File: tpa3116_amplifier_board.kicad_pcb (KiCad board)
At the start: 2 copper layers, 60.3 x 50.8 mm, 41 parts, among them IC1 TPA3116D2QDADRQ1, J1 power_supply, J2 Conn_01x04, J3 power_supply, J4 output_right

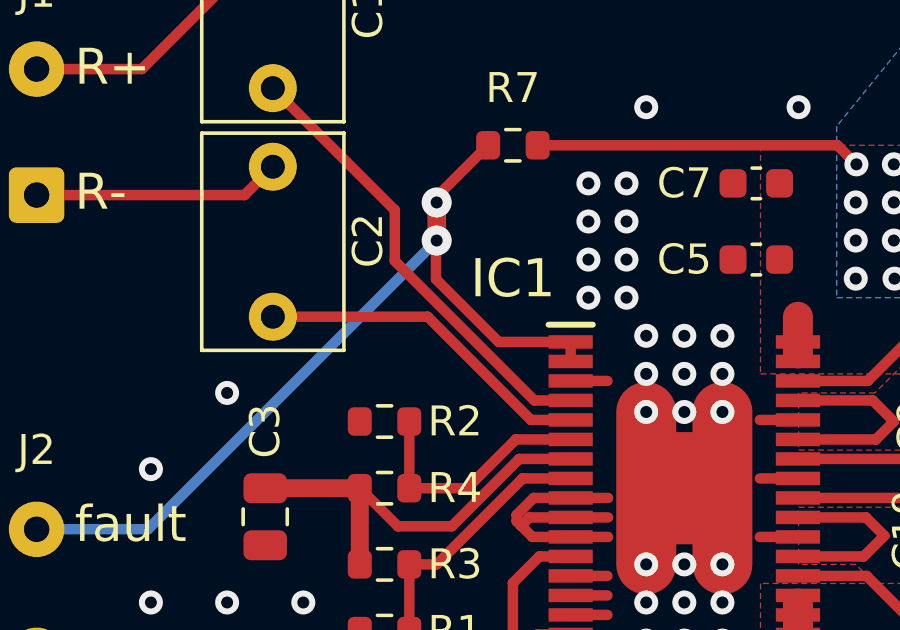
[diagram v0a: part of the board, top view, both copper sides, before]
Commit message: исправил ошибку в схеме
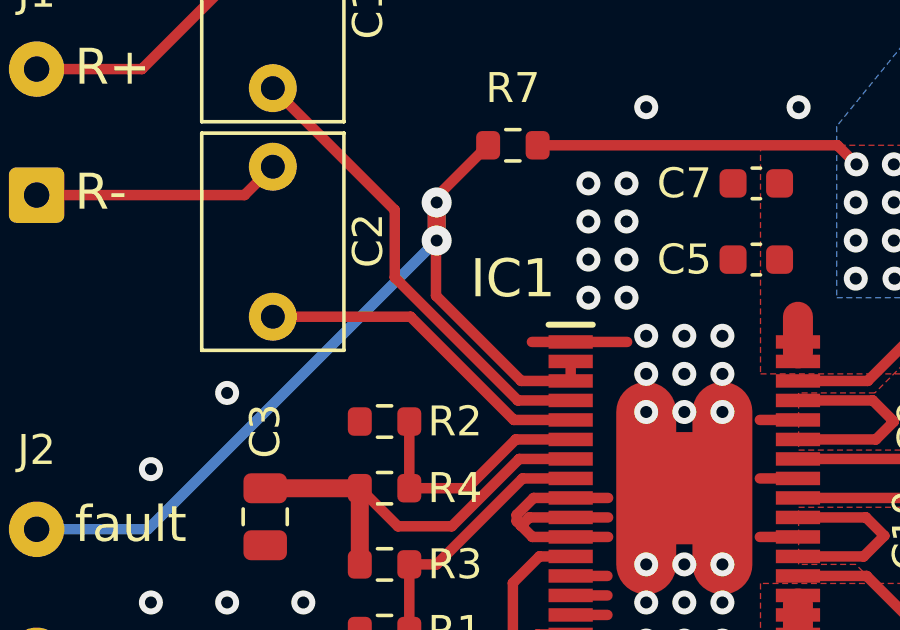
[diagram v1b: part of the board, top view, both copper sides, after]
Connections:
- IC1 pad 1: /SD_LR -> GND
- IC1 pad 3: GND -> /SD_LR
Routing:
- net GND: track 35.0 -> 36.9 mm
- net /SD_LR: track 29.8 -> 30.6 mm
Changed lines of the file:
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@@
       (stroke (width 0.1) (type solid)) (layer "F.Fab"))
     (pad "1" smd rect (at -3.788 -4.875 90) (size 0.45 1.475) (layers "F.Cu" "F.Paste" "F.Mask")
-      (net 16 "/SD_LR") (pinfunction "MODSEL") (pintype "passive"))
+      (net 5 "GND") (pinfunction "MODSEL") (pintype "passive"))
     (pad "2" smd rect (at -3.788 -4.225 90) (size 0.45 1.475) (layers "F.Cu" "F.Paste" "F.Mask")
       (net 16 "/SD_LR") (pinfunction "SD") (pintype "passive"))
     (pad "3" smd rect (at -3.788 -3.575 90) (size 0.45 1.475) (layers "F.Cu" "F.Paste" "F.Mask")
-      (net 5 "GND") (pinfunction "FAULT") (pintype "passive"))
+      (net 16 "/SD_LR") (pinfunction "FAULT") (pintype "passive"))
     (pad "4" smd rect (at -3.788 -2.925 90) (size 0.45 1.475) (layers "F.Cu" "F.Paste" "F.Mask")
       (net 2 "Net-(IC1-RINP)") (pinfunction "RINP") (pintype "passive"))
@@
   (segment (start 106.379 106.045) (end 102.87 106.045) (width 0.35) (layer "F.Cu") (net 1))
   (segment (start 110.744 101.68) (end 106.379 106.045) (width 0.35) (layer "F.Cu") (net 1))
-  (segment (start 120.672 117.09) (end 119.459831 117.09) (width 0.35) (layer "F.Cu") (net 2))
-  (segment (start 114.808 112.438169) (end 114.808 110.744) (width 0.35) (layer "F.Cu") (net 2))
-  (segment (start 119.459831 117.09) (end 114.808 112.438169) (width 0.35) (layer "F.Cu") (net 2))
+  (segment (start 118.909915 117.09) (end 114.808 112.988085) (width 0.35) (layer "F.Cu") (net 2))
   (segment (start 114.808 110.744) (end 110.744 106.68) (width 0.35) (layer "F.Cu") (net 2))
+  (segment (start 120.672 117.09) (end 118.909915 117.09) (width 0.35) (layer "F.Cu") (net 2))
+  (segment (start 114.808 112.988085) (end 114.808 110.744) (width 0.35) (layer "F.Cu") (net 2))
   (segment (start 102.87 110.245) (end 109.799 110.245) (width 0.35) (layer "F.Cu") (net 3))
   (segment (start 109.799 110.245) (end 110.744 109.3) (width 0.35) (layer "F.Cu") (net 3))
-  (segment (start 119.346155 117.74) (end 115.906155 114.3) (width 0.35) (layer "F.Cu") (net 4))
-  (segment (start 120.672 117.74) (end 119.346155 117.74) (width 0.35) (layer "F.Cu") (net 4))
-  (segment (start 115.906155 114.3) (end 110.744 114.3) (width 0.35) (layer "F.Cu") (net 4))
+  (segment (start 118.776538 117.74) (end 115.336538 114.3) (width 0.35) (layer "F.Cu") (net 4))
+  (segment (start 120.672 117.74) (end 118.776538 117.74) (width 0.35) (layer "F.Cu") (net 4))
+  (segment (start 115.336538 114.3) (end 110.744 114.3) (width 0.35) (layer "F.Cu") (net 4))
   (segment (start 128.248 119.69) (end 126.978 119.69) (width 0.35) (layer "F.Cu") (net 5))
   (segment (start 120.672 122.94) (end 121.898 122.94) (width 0.35) (layer "F.Cu") (net 5))
@@
   (segment (start 128.248 121.64) (end 126.978 121.64) (width 0.35) (layer "F.Cu") (net 5))
   (segment (start 120.672 124.24) (end 121.898 124.24) (width 0.35) (layer "F.Cu") (net 5))
-  (segment (start 120.672 116.44) (end 121.898 116.44) (width 0.35) (layer "F.Cu") (net 5))
   (segment (start 120.672 121.64) (end 121.92 121.64) (width 0.35) (layer "F.Cu") (net 5))
   (segment (start 120.672 120.34) (end 121.92 120.34) (width 0.35) (layer "F.Cu") (net 5))
@@
   (segment (start 119.0195 121.2645) (end 119.395 121.64) (width 0.35) (layer "F.Cu") (net 5))
   (segment (start 119.395 121.64) (end 120.672 121.64) (width 0.35) (layer "F.Cu") (net 5))
+  (segment (start 119.38 115.14) (end 122.555 115.14) (width 0.35) (layer "F.Cu") (net 5))
   (segment (start 120.672 120.99) (end 121.92 120.99) (width 0.35) (layer "F.Cu") (net 5))
   (segment (start 119.436 120.34) (end 118.872 120.904) (width 0.35) (layer "F.Cu") (net 5))
@@
   (segment (start 128.248 122.94) (end 130.538 122.94) (width 0.35) (layer "F.Cu") (net 15))
   (segment (start 132.058 124.46) (end 132.058 125.708) (width 0.35) (layer "F.Cu") (net 15))
-  (segment (start 118.273507 115.14) (end 120.672 115.14) (width 0.35) (layer "F.Cu") (net 16))
   (segment (start 116.205 110.3) (end 116.205 110.49) (width 0.35) (layer "F.Cu") (net 16))
+  (segment (start 116.183 111.782) (end 116.183 113.599409) (width 0.35) (layer "F.Cu") (net 16))
+  (segment (start 120.672 116.44) (end 120.672 115.79) (width 0.35) (layer "F.Cu") (net 16))
+  (segment (start 119.023591 116.44) (end 120.672 116.44) (width 0.35) (layer "F.Cu") (net 16))
+  (segment (start 116.205 110.49) (end 116.205 111.76) (width 0.6) (layer "F.Cu") (net 16))
   (segment (start 116.205 111.76) (end 116.183 111.782) (width 0.35) (layer "F.Cu") (net 16))
-  (segment (start 120.672 115.79) (end 120.672 115.14) (width 0.35) (layer "F.Cu") (net 16))
-  (segment (start 116.183 113.049493) (end 118.273507 115.14) (width 0.35) (layer "F.Cu") (net 16))
-  (segment (start 116.205 110.49) (end 116.205 111.76) (width 0.6) (layer "F.Cu") (net 16))
-  (segment (start 116.183 111.782) (end 116.183 113.049493) (width 0.35) (layer "F.Cu") (net 16))
+  (segment (start 116.183 113.599409) (end 119.023591 116.44) (width 0.35) (layer "F.Cu") (net 16))
   (segment (start 117.92 108.585) (end 116.205 110.3) (width 0.35) (layer "F.Cu") (net 16))
   (via (at 116.205 110.49) (size 1) (drill 0.4) (layers "F.Cu" "B.Cu") (net 16))
